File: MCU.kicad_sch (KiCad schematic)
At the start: 31 parts, among them SW1 SW_Reed, U4 STM32U595RITx, U8 ATECC608A-SSHDA, X1 SMD3225-4, X2 SMD2012-2

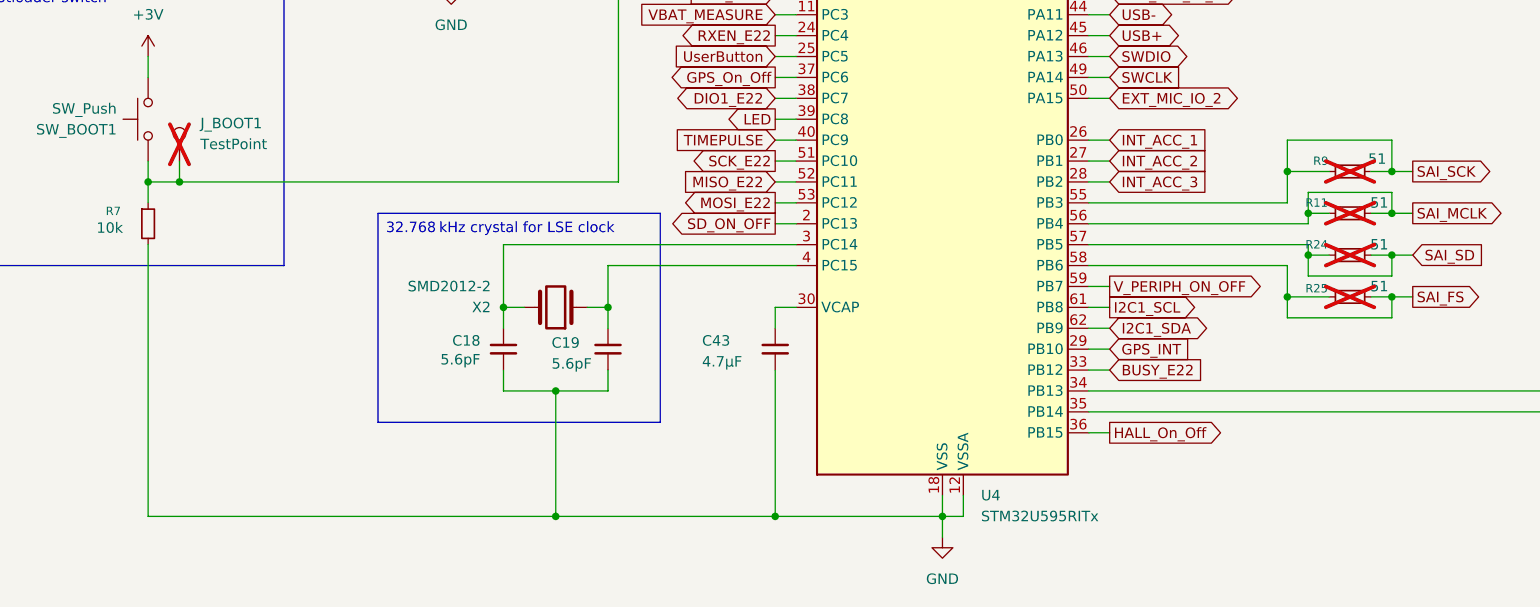
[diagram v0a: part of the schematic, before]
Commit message: WIP: BOM
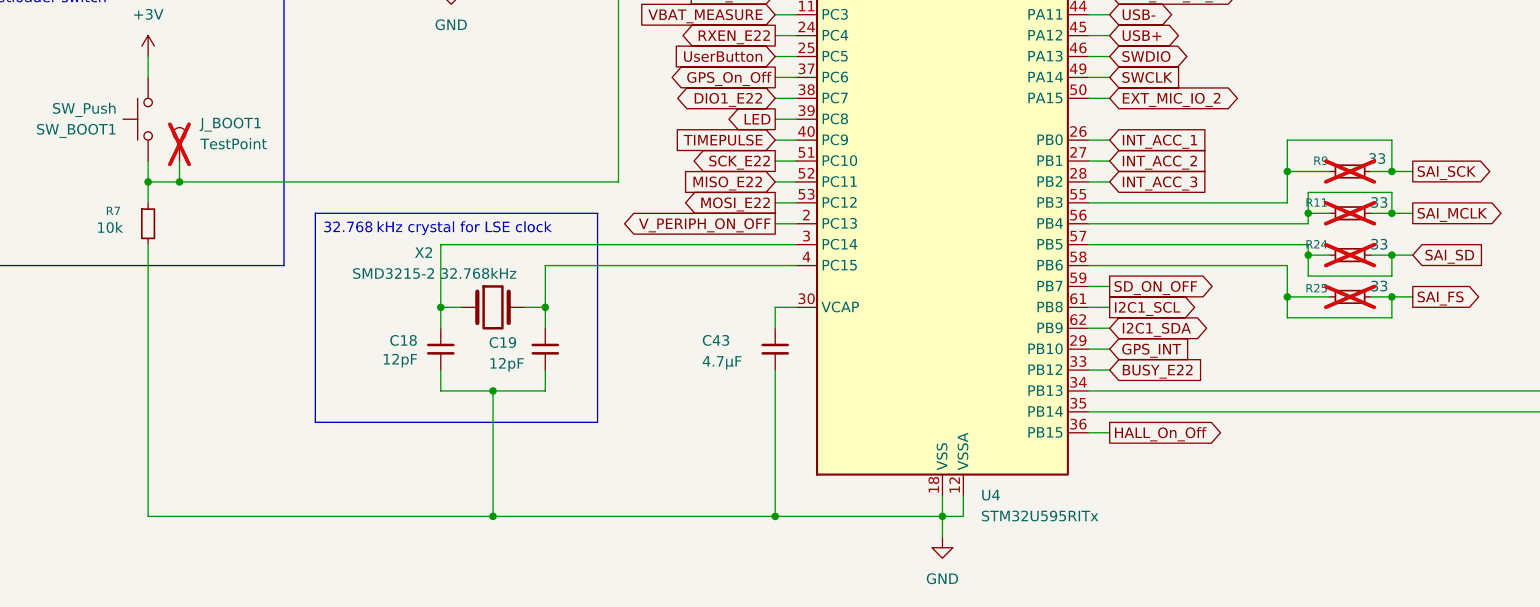
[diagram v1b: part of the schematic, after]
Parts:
- removed X2: SMD2012-2, PCM_Crystal_AKL:Crystal_SMD_2012-2Pin_2.0x1.2mm, symbol PCM_Crystal_AKL:SMD2012-2
- added X2: SMD3215-2 32.768kHz, PCM_Crystal_AKL:Crystal_SMD_3215-2Pin_3.2x1.5mm, symbol PCM_Crystal_AKL:SMD3215-2
- C11, C3, C43, C7: LCSC (none) -> C23733
- C12, C13, C4, C5, C6: LCSC (none) -> C1525
- C14, C15: LCSC (none) -> C1547
- C18, C19: value 5.6pF -> 12pF; LCSC (none) -> C1547
- C25: LCSC (none) -> C1525; now left out of the parts list
- C8: LCSC (none) -> C15195
- R11, R24, R25, R9: value 51 -> 33; LCSC (none) -> C25105
- R13, R14: LCSC (none) -> C25900
- R7: LCSC (none) -> C25744
- SW_BOOT1, SW_RST1: LCSC (none) -> C223812
- U4: LCSC (none) -> C28563722; LCSC Old (none) -> C28247611
- U8: LCSC (none) -> C616024
- X1: LCSC (none) -> C13738
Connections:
- net SD_ON_OFF: now also U4.59 (PB7); no longer U4.2 (PC13)
- net V_PERIPH_ON_OFF: now also U4.2 (PC13); no longer U4.59 (PB7)
- net at C18.1, U4.3 (PC14): now also X2.1
- net at C19.1, U4.4 (PC15): now also X2.2
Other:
- moved on the sheet: C18, C19

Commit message: Finish routing + silkscreen placement
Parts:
- SW_BOOT1, SW_RST1: FT Rotation Offset (none) -> 180
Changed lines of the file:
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@@
+			)
+		)
+		(property "FT Rotation Offset" "180"
+			(at 40.64 63.5 90)
+			(hide yes)
+			(show_name no)
+			(do_not_autoplace no)
+			(effects
+				(font
+					(size 1.27 1.27)
+				)
 			)
 		)
@@
 			(at 36.83 96.52 90)
 			(hide yes)
+			(show_name no)
+			(do_not_autoplace no)
+			(effects
+				(font
+					(size 1.27 1.27)
+				)
+			)
+		)
+		(property "FT Rotation Offset" "180"
+			(at 36.83 96.52 90)
+			(hide yes)
